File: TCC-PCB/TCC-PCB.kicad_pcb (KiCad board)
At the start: 2 copper layers, 1 part, among them U1 ATmega32U4-A

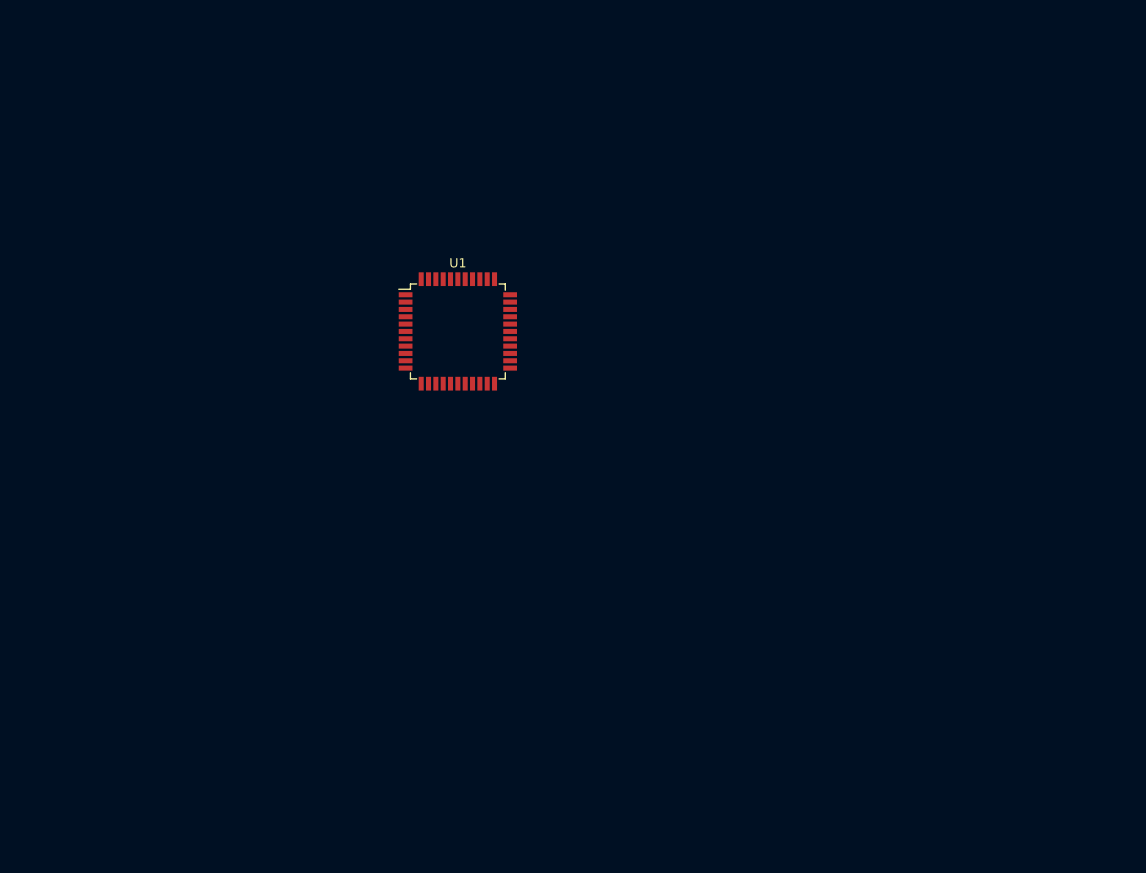
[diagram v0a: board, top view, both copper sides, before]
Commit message: changes
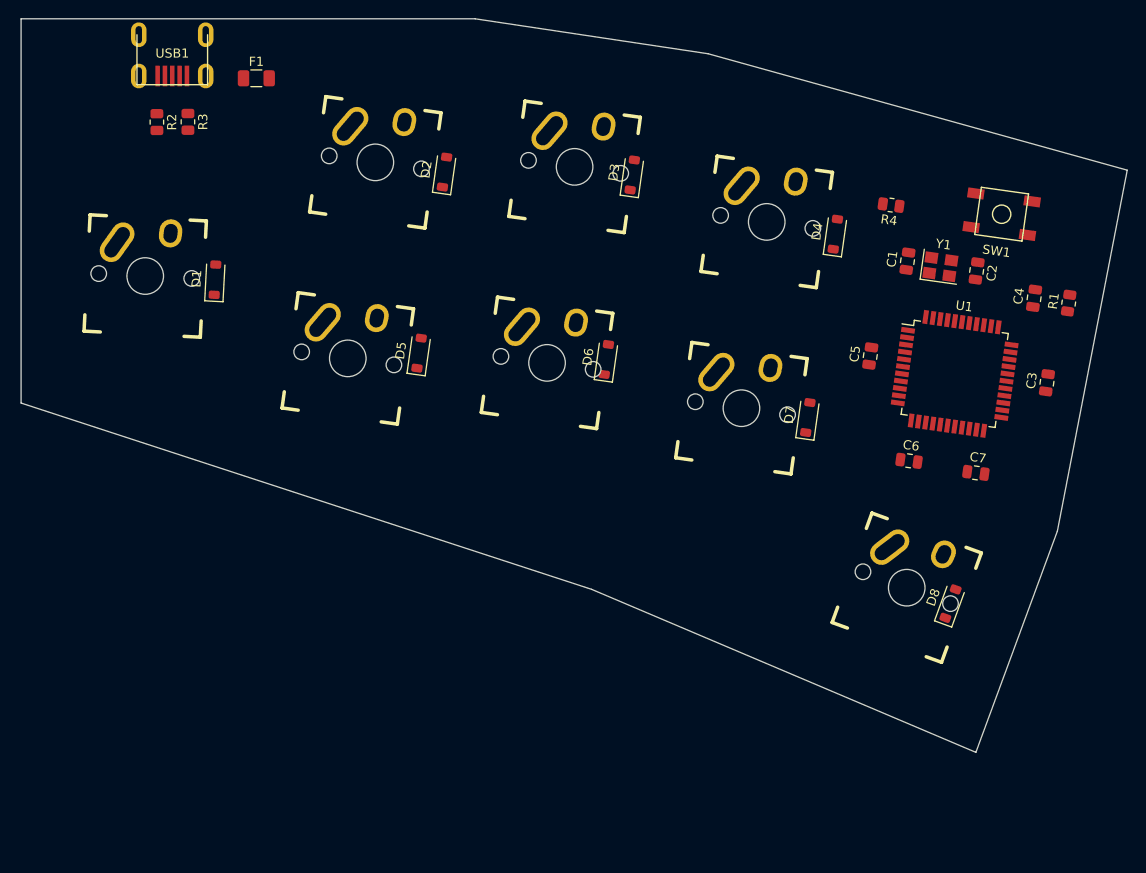
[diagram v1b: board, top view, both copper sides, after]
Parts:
- added C1: 1uf, Capacitor_SMD:C_0805_2012Metric, F.Cu at (188.1, 74.7)
- added C2: 0.1uF, Capacitor_SMD:C_0805_2012Metric, F.Cu at (195.7, 75.8)
- added C3: 0.1uF, Capacitor_SMD:C_0805_2012Metric, F.Cu at (203.3, 88.0)
- added C4: 0.1uF, Capacitor_SMD:C_0805_2012Metric, F.Cu at (201.9, 78.7)
- added C5: 10uF, Capacitor_SMD:C_0805_2012Metric, F.Cu at (184.1, 85.0)
- added C6: 22pF, Capacitor_SMD:C_0805_2012Metric, F.Cu at (188.3, 96.5)
- added C7: 22pF, Capacitor_SMD:C_0805_2012Metric, F.Cu at (195.6, 97.8)
- added D1: SOD-123, Diode_SMD:D_SOD-123, F.Cu at (112.6, 76.7)
- added D2: SOD-123, Diode_SMD:D_SOD-123, F.Cu at (137.6, 65.0)
- added D3: SOD-123, Diode_SMD:D_SOD-123, F.Cu at (158.1, 65.3)
- added D4: SOD-123, Diode_SMD:D_SOD-123, F.Cu at (180.2, 71.8)
- added D5: SOD-123, Diode_SMD:D_SOD-123, F.Cu at (134.8, 84.7)
- added D6: SOD-123, Diode_SMD:D_SOD-123, F.Cu at (155.3, 85.4)
- added D7: SOD-123, Diode_SMD:D_SOD-123, F.Cu at (177.2, 91.8)
- added D8: SOD-123, Diode_SMD:D_SOD-123, F.Cu at (192.8, 112.0)
- added F1: Polyfuse, Fuse:Fuse_1206_3216Metric, F.Cu at (117.1, 54.8)
- added MX1: MX-NoLED, keebs:Mx_Alps_100, F.Cu at (105.0, 76.3)
- added MX2: MX-NoLED, keebs:Mx_Alps_100, F.Cu at (130.1, 63.9)
- added MX3: MX-NoLED, keebs:Mx_Alps_100, F.Cu at (151.8, 64.4)
- added MX4: MX-NoLED, keebs:Mx_Alps_100, F.Cu at (172.8, 70.4)
- added MX5: MX-NoLED, keebs:Mx_Alps_100, F.Cu at (127.1, 85.3)
- added MX6: MX-NoLED, keebs:Mx_Alps_100, F.Cu at (148.8, 85.8)
- added MX7: MX-NoLED, keebs:Mx_Alps_100, F.Cu at (170.0, 90.7)
- added MX8: MX-NoLED, keebs:Mx_Alps_100, F.Cu at (188.0, 110.3)
- added R1: 10k, Resistor_SMD:R_0805_2012Metric, F.Cu at (205.7, 79.3)
- added R2: 22, Resistor_SMD:R_0805_2012Metric, F.Cu at (106.2, 59.5)
- added R3: 22, Resistor_SMD:R_0805_2012Metric, F.Cu at (109.6, 59.5)
- added R4: R_Small, Resistor_SMD:R_0805_2012Metric, F.Cu at (186.3, 68.6)
- added SW1: SW_Push, random-keyboard-parts:SKQG-1155865, F.Cu at (198.4, 69.6)
- added USB1: Molex-0548190589, random-keyboard-parts:Molex-0548190589, F.Cu at (107.9, 50.0)
- added Y1: Crystal_GND24_Small, Crystal:Crystal_SMD_3225-4Pin_3.2x2.5mm, F.Cu at (191.7, 75.3)
- moved U1 54.4 mm to (193.3, 87.0), turned to -8 degrees
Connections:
- U1 pad 26: unconnected-(U1-PD6-Pad26) -> ROW1
- U1 pad 30: ROW1 -> COL2
- U1 pad 31: unconnected-(U1-PC6-Pad31) -> COL3
- U1 pad 32: unconnected-(U1-PC7-Pad32) -> COL4
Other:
- board outline added: 120.7 x 80 mm

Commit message: name change
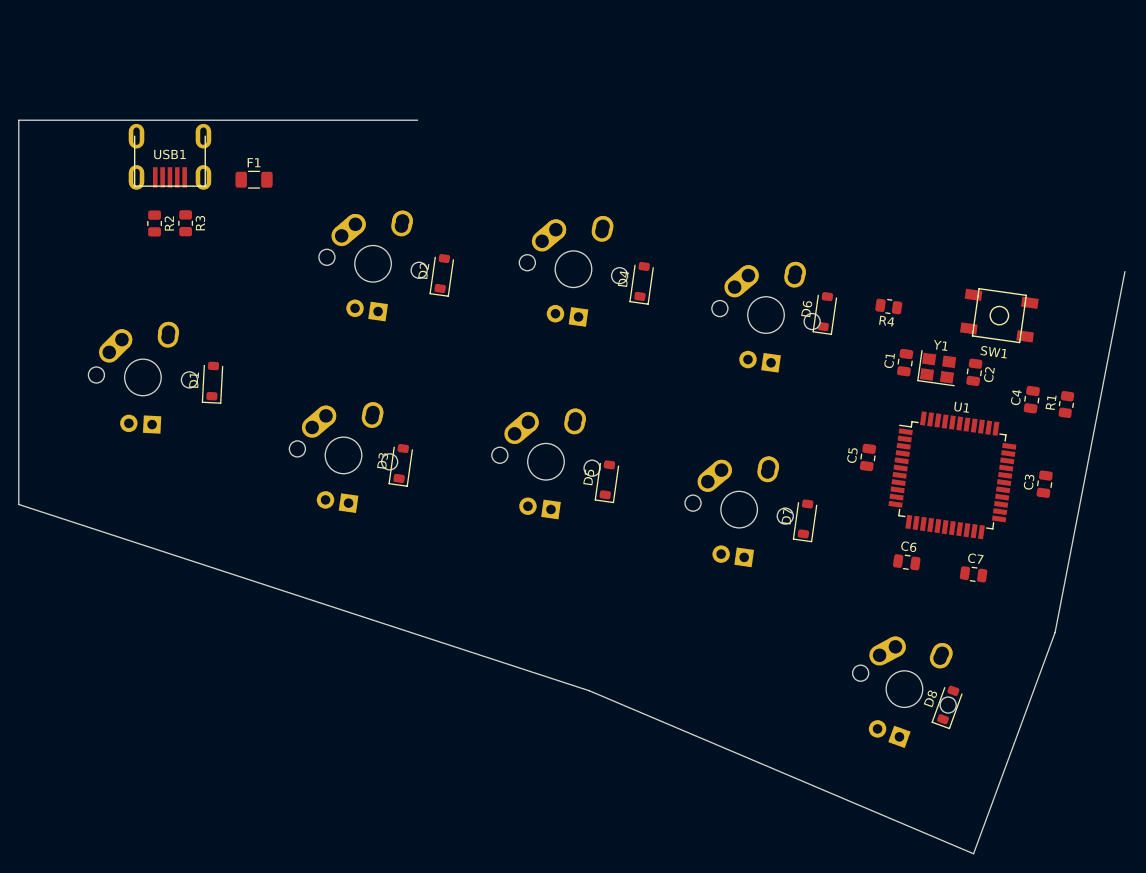
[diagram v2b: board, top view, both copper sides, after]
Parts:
- MX1, MX2, MX3, MX4, MX5, MX6, MX7, MX8: footprint keebs:Mx_Alps_100 -> MX_Alps_Hybrid:MX-1U
- moved D3 40.3 mm to (132.9, 96.8)
- moved MX3 40.3 mm to (126.6, 95.9)
- moved D5 24.8 mm to (155.4, 98.5)
- moved D6 24.4 mm to (179.2, 80.2)
- moved MX6 24.4 mm to (172.7, 80.6)
- moved MX5 24.4 mm to (148.7, 96.6)
- moved MX4 21.7 mm to (151.7, 75.6)
- moved D4 21.7 mm to (159.2, 76.9)
- moved R2 11.1 mm to (106.0, 70.6)
- moved C1 11.1 mm to (187.9, 85.8)
- moved C2 11.1 mm to (195.4, 86.8)
- moved C3 11.1 mm to (203.1, 99.0)
- moved C4 11.1 mm to (201.7, 89.8)
- moved C5 11.1 mm to (183.8, 96.1)
- moved C6 11.1 mm to (188.0, 107.5)
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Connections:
- D2 pad 1: Net-(D1-K) -> Net-(D2-K)
- D3 pad 1: Net-(D3-K) -> Net-(D1-K)
- D4 pad 1: Net-(D3-K) -> Net-(D2-K)
- D6 pad 1: Net-(D1-K) -> Net-(D2-K)
- D7 pad 1: Net-(D3-K) -> Net-(D1-K)
- D8 pad 1: Net-(D3-K) -> Net-(D2-K)
- MX3 pad 1: COL2 -> COL1
- MX3 pad 2: Net-(D5-A) -> Net-(D3-A)
- MX4 pad 1: COL3 -> COL2
- MX4 pad 2: Net-(D6-A) -> Net-(D4-A)
- MX5 pad 1: COL1 -> COL2
- MX5 pad 2: Net-(D3-A) -> Net-(D5-A)
- MX6 pad 1: COL2 -> COL3
- MX6 pad 2: Net-(D4-A) -> Net-(D6-A)
- MX8 pad 1: COL3 -> COL4
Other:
- outline, holes or cut-outs redrawn

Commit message: updates and used footprints
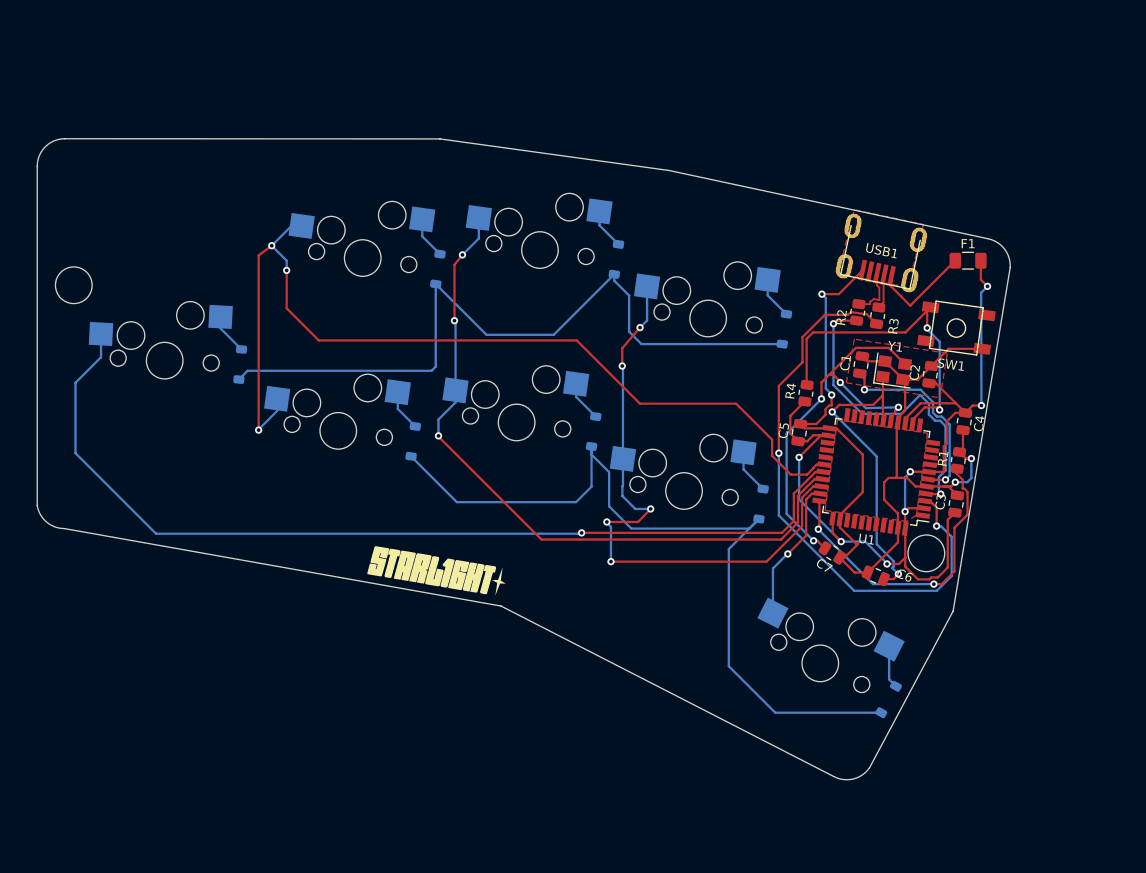
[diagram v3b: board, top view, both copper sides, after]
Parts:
- added G***: LOGO, TCC-PCB:logo, F.Cu at (136.7, 108.5)
- D1, D2, D3, D4, D5, D6, D7, D8: moved to B.Cu
- MX1, MX2, MX3, MX4, MX5, MX6, MX7, MX8: footprint MX_Alps_Hybrid:MX-1U -> MX_Only:MXOnly-1U-Hotswap
- moved USB1 78.8 mm to (185.7, 71.6), turned to -102 degrees
- moved F1 78.4 mm to (194.7, 74.6)
- moved R2 77.3 mm to (182.7, 80.3), turned to -98 degrees
- moved R3 76.2 mm to (184.9, 80.6), turned to -98 degrees
- moved D5 24.1 mm to (156.4, 74.5)
- moved MX5 23.1 mm to (148.0, 73.5)
- moved D6 22.1 mm to (172.2, 101.2)
- moved MX3 21.6 mm to (128.7, 74.4)
- moved D3 21.6 mm to (136.9, 75.6)
- moved MX6 21.2 mm to (163.7, 99.8)
- moved MX7 21.1 mm to (166.4, 81.0)
- moved D7 20.8 mm to (174.7, 82.1)
- moved MX2 18.6 mm to (126.0, 93.2)
- moved D2 18.6 mm to (134.2, 94.4)
- moved MX4 17.8 mm to (145.5, 92.3)
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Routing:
- net GND: track 0.00 -> 106.3 mm, vias 0 -> 4
- net COL1: track 0.00 -> 104.5 mm, vias 0 -> 3
- net COL0: track 0.00 -> 104.2 mm, vias 0 -> 1
- net +5V: track 0.00 -> 102.1 mm, vias 0 -> 7
- net Net-(D2-K): track 0.00 -> 88.1 mm
- net Net-(D1-K): track 0.00 -> 79.8 mm
- net COL2: track 0.00 -> 76.7 mm, vias 0 -> 3
- net COL3: track 0.00 -> 65.8 mm, vias 0 -> 5
- net Net-(U1-D-): track 0.00 -> 63.0 mm, vias 0 -> 2
- net Net-(U1-XTAL2): track 0.00 -> 44.4 mm, vias 0 -> 4
- net Net-(U1-~{RESET}): track 0.00 -> 36.3 mm, vias 0 -> 2
- net Net-(U1-D+): track 0.00 -> 35.2 mm, vias 0 -> 2
- net Net-(U1-XTAL1): track 0.00 -> 33.9 mm, vias 0 -> 2
- net Net-(U1-~{HWB}/PE2): track 0.00 -> 33.6 mm, vias 0 -> 2
- net Net-(U1-UCAP): track 0.00 -> 21.7 mm, vias 0 -> 2
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- added copper zone on F.Cu, net (none)
- added copper zone on F.Cu, net GND
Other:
- board size 120.7 x 80 mm -> 106.1 x 69.9 mm

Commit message: final changes
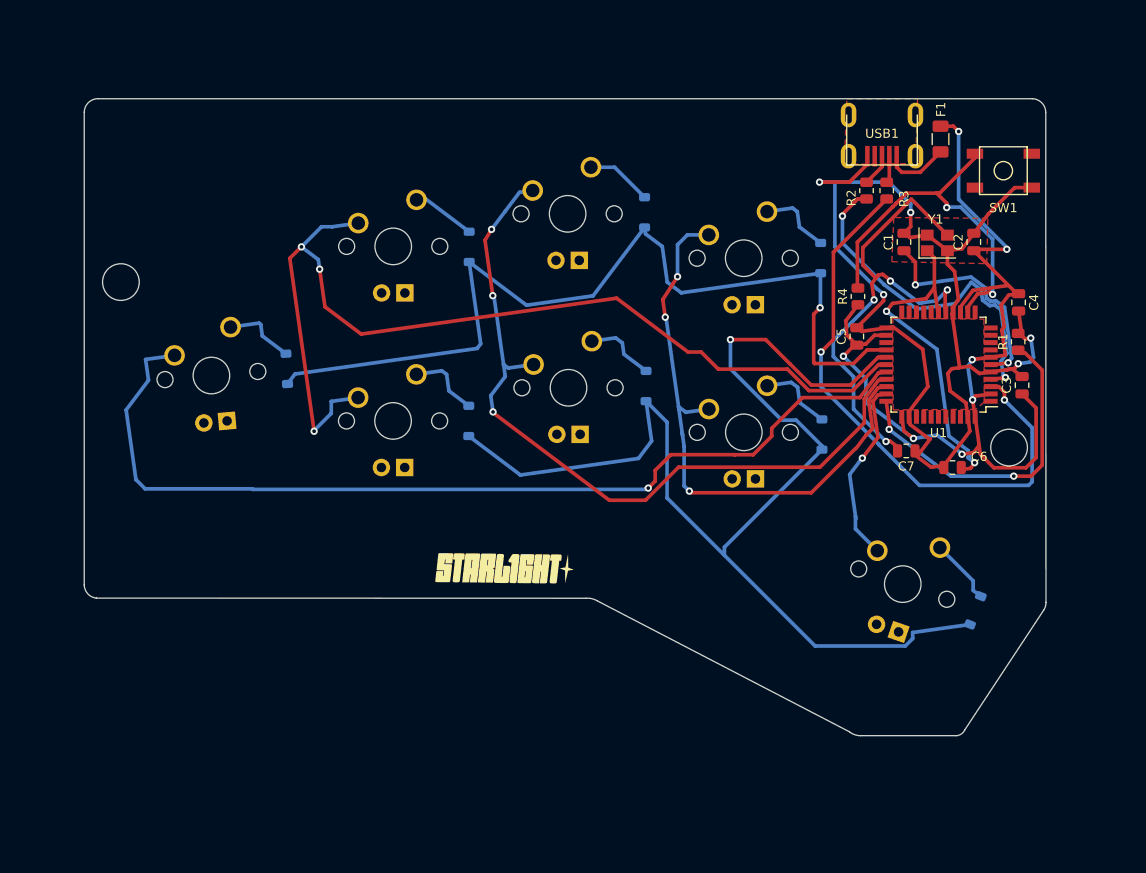
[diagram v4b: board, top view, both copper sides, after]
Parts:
- MX1, MX2, MX3, MX4, MX5, MX6, MX7, MX8: footprint MX_Only:MXOnly-1U-Hotswap -> MX_Only:MXOnly-1U
- moved SW1 17.9 mm to (198.6, 64.8), turned to 0 degrees
- moved C2 15.2 mm to (195.4, 72.6), turned to 90 degrees
- moved C3 14.8 mm to (200.6, 88.2), turned to 90 degrees
- moved Y1 14.7 mm to (191.4, 72.7), turned to 0 degrees
- moved R1 14.5 mm to (200.2, 83.5), turned to 90 degrees
- moved C6 14.5 mm to (193.0, 97.2), turned to 0 degrees
- moved C4 14.3 mm to (200.2, 79.2), turned to -90 degrees
- moved C1 14.2 mm to (187.7, 72.6), turned to 90 degrees
- moved C7 13.7 mm to (188.0, 95.4), turned to 180 degrees
- moved R3 13.7 mm to (185.9, 67.0), turned to -90 degrees
- moved F1 13.6 mm to (191.7, 61.4), turned to 90 degrees
- moved D8 13.6 mm to (195.5, 112.8), turned to 69 degrees
- moved U1 13.5 mm to (191.5, 86.0), turned to 180 degrees
- moved R2 13.3 mm to (183.7, 67.0), turned to -90 degrees
- moved USB1 12.9 mm to (185.3, 58.8), turned to -90 degrees
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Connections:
- D1 pad 1: Net-(D1-K) -> ROW0
- D2 pad 1: Net-(D2-K) -> ROW1
- D3 pad 1: Net-(D1-K) -> ROW0
- D4 pad 1: Net-(D2-K) -> ROW1
- D5 pad 1: Net-(D1-K) -> ROW0
- D6 pad 1: Net-(D2-K) -> ROW1
- D7 pad 1: Net-(D1-K) -> ROW0
- D8 pad 1: Net-(D2-K) -> ROW1
- U1 pad 26: ROW1 -> ROW0
- U1 pad 27: ROW0 -> ROW1
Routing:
- net ROW1: track 0.00 -> 132.5 mm, vias 0 -> 1
- net ROW0: track 0.00 -> 98.4 mm, vias 0 -> 1
- net Net-(D2-K): track 88.1 -> 0.00 mm
- net Net-(D1-K): track 79.8 -> 0.00 mm
- net GND: track 106.3 -> 127.8 mm, vias 4 -> 5
- net Net-(U1-XTAL2): track 44.4 -> 53.2 mm
- net COL2: track 76.7 -> 84.1 mm
- net +5V: track 102.1 -> 108.9 mm
- net COL1: track 104.5 -> 109.9 mm
- net COL4: track 15.7 -> 20.5 mm
- net Net-(U1-~{RESET}): track 36.3 -> 40.8 mm
- net VCC: track 11.0 -> 7.13 mm
- net Net-(U1-D+): track 35.2 -> 39.1 mm
- net Net-(D7-A): track 4.59 -> 8.05 mm
- net Net-(D2-A): track 4.52 -> 7.98 mm
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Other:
- board size 106.1 x 69.9 mm -> 104.9 x 69.5 mm
